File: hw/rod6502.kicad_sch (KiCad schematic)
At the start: 4 parts, among them J1 Conn_01x08_Socket, J2 Conn_01x08_Socket, U1 W65C02SxP

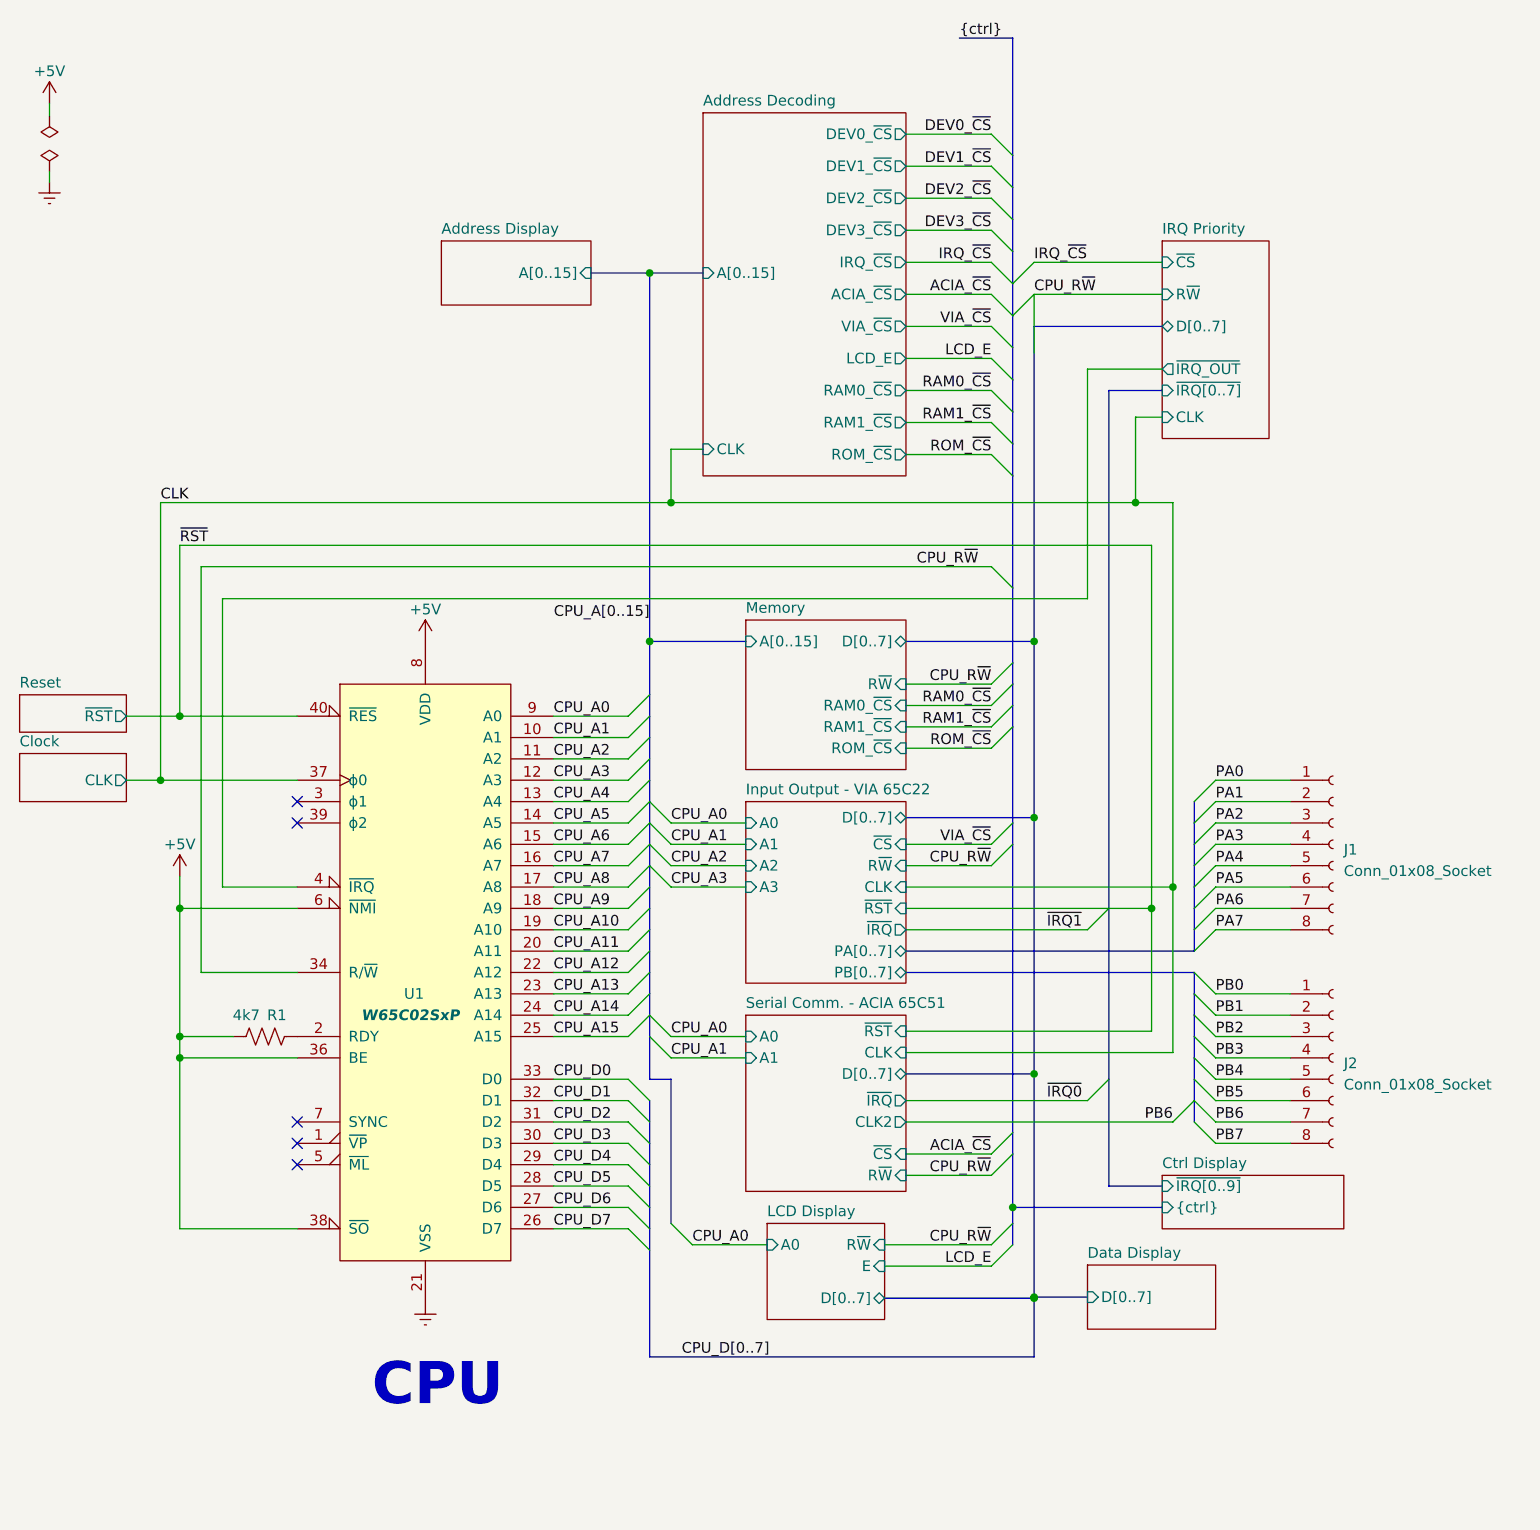
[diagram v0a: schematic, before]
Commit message: add hw design for veraduino
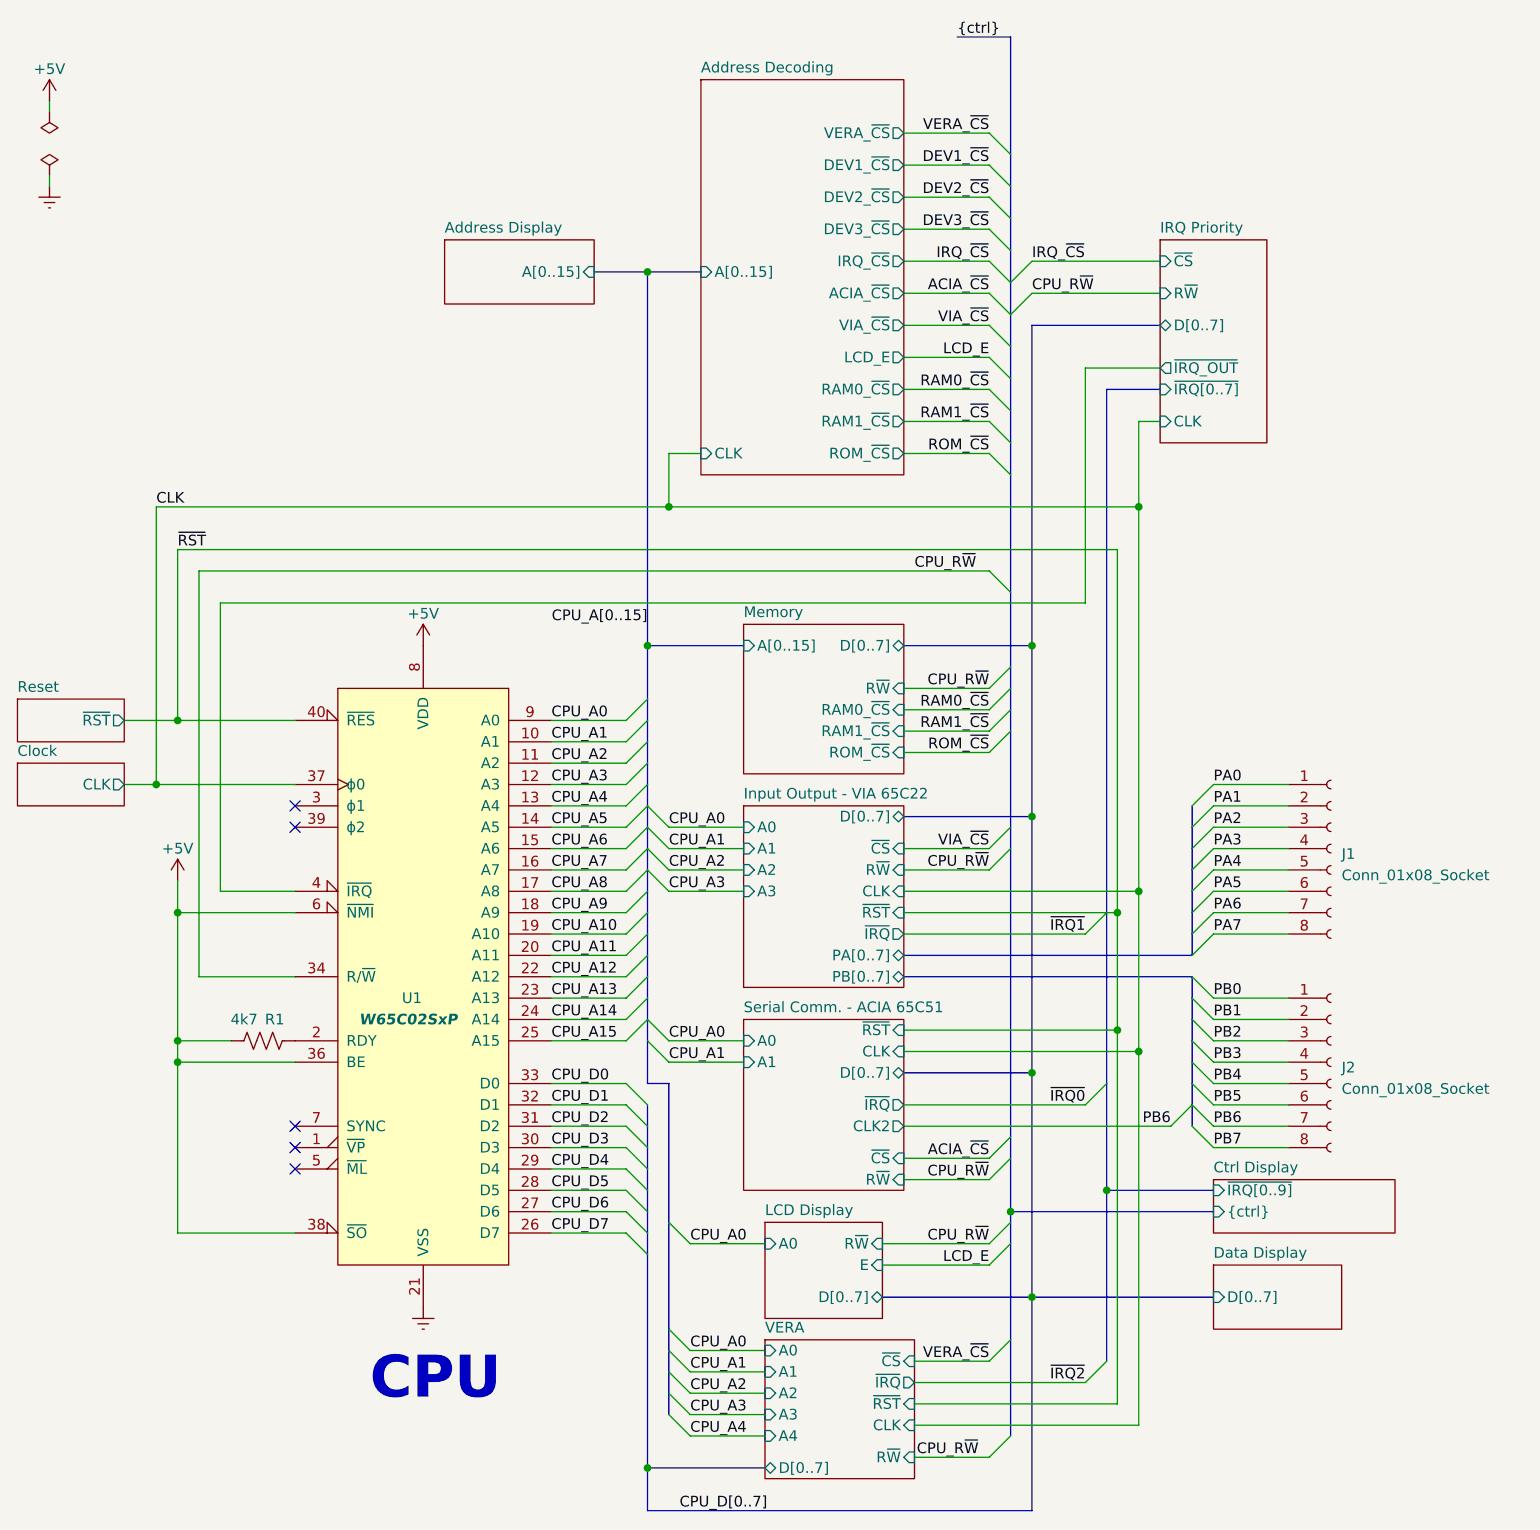
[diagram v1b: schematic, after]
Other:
- added sheet VERA (vera.kicad_sch.kicad_sch)
- sheet Address Decoding ports: added VERA_~{CS}; removed DEV0_~{CS}
- moved on the sheet: J1, J2, R1, U1

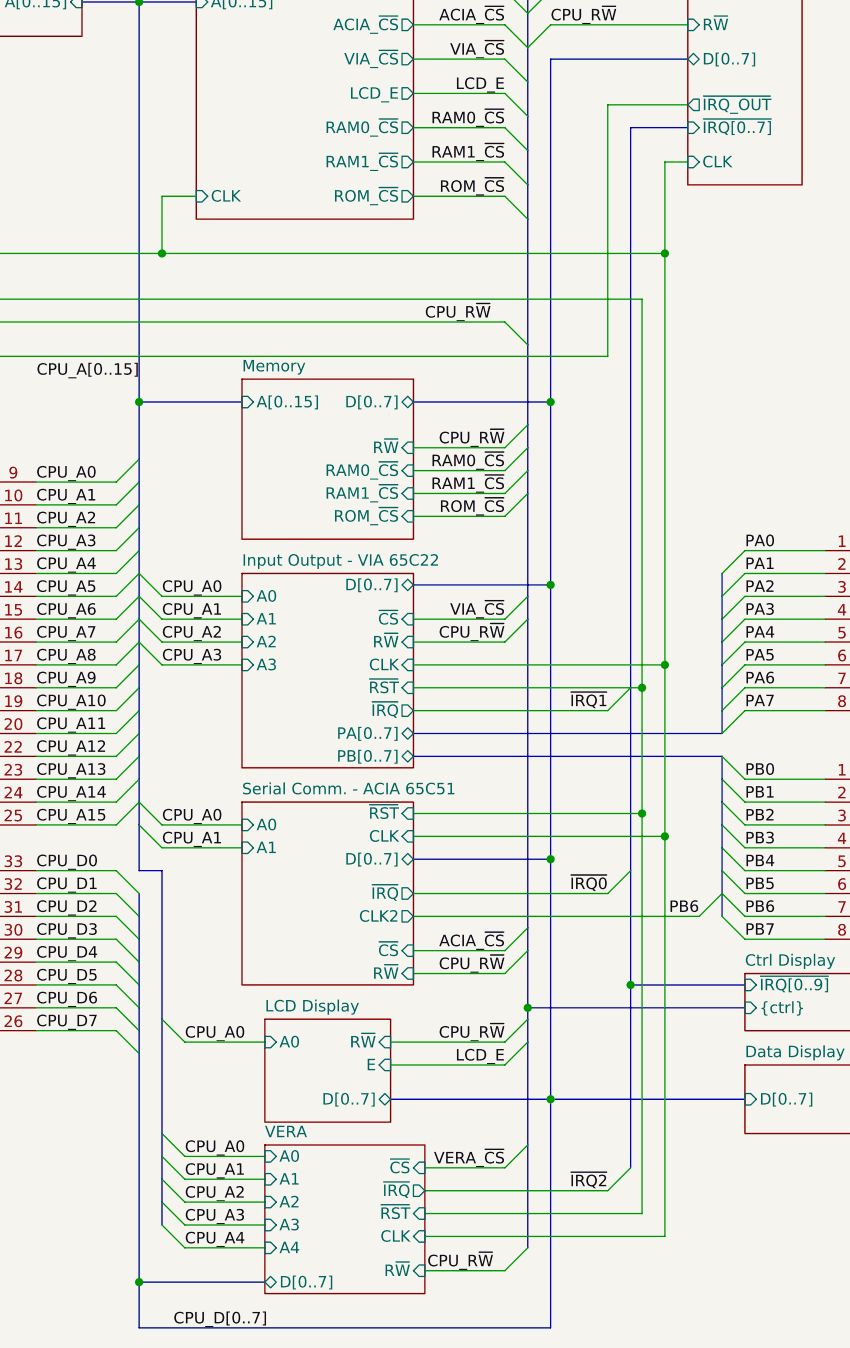
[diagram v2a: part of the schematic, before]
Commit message: clean up hw schematics
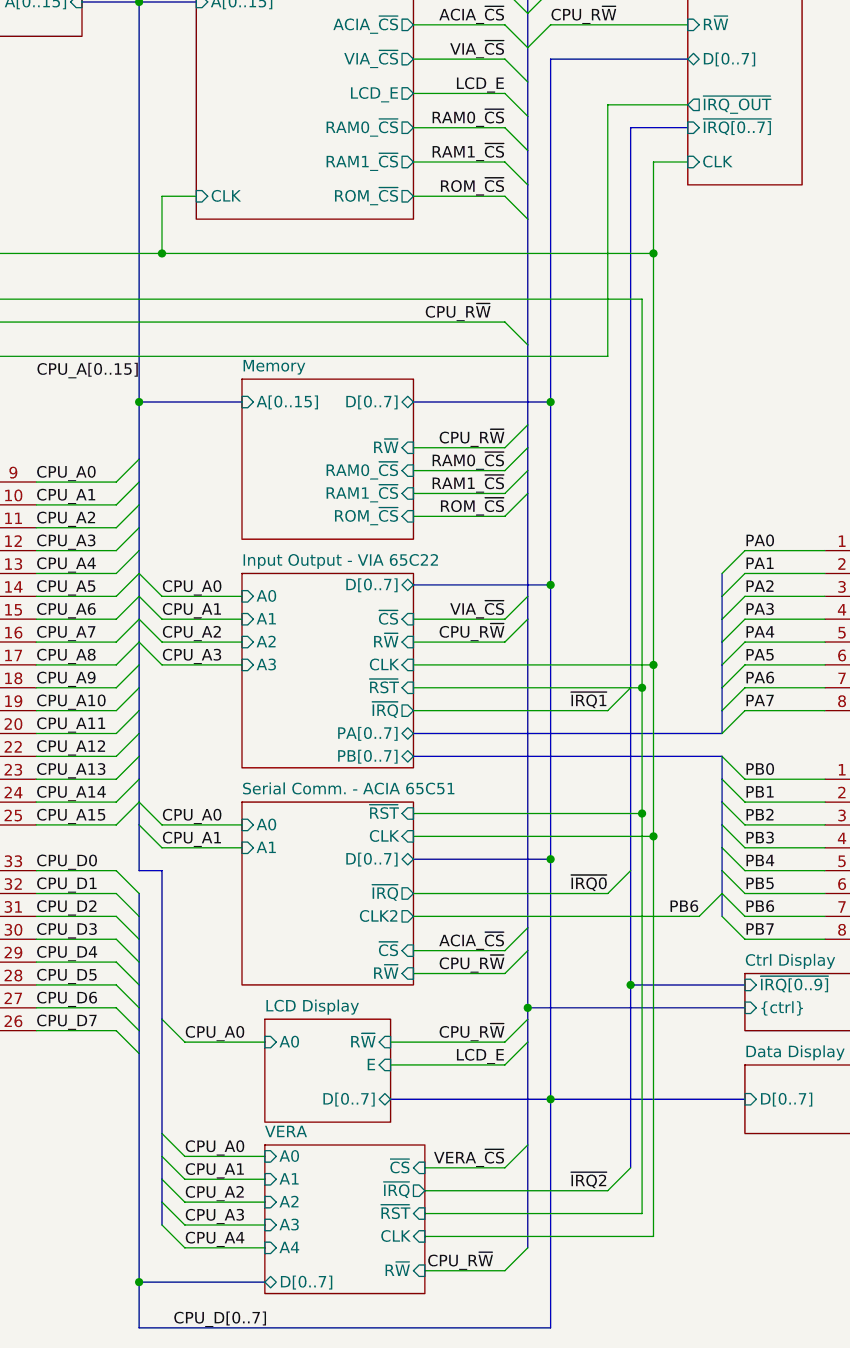
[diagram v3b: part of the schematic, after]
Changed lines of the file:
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@@
   (junction (at 137.16 88.9) (diameter 0) (color 0 0 0 0)
   )
+  (junction (at 148.59 72.39) (diameter 0) (color 0 0 0 0)
+  )
   (junction (at 35.56 120.65) (diameter 0) (color 0 0 0 0)
   )
@@
   (junction (at 91.44 88.9) (diameter 0) (color 0 0 0 0)
   )
+  (junction (at 148.59 118.11) (diameter 0) (color 0 0 0 0)
+  )
   (junction (at 137.16 139.7) (diameter 0) (color 0 0 0 0)
   )
@@
   (junction (at 137.16 166.37) (diameter 0) (color 0 0 0 0)
   )
+  (junction (at 148.59 137.16) (diameter 0) (color 0 0 0 0)
+  )
   (junction (at 147.32 120.65) (diameter 0) (color 0 0 0 0)
-  )
-  (junction (at 149.86 137.16) (diameter 0) (color 0 0 0 0)
-  )
-  (junction (at 149.86 118.11) (diameter 0) (color 0 0 0 0)
-  )
-  (junction (at 149.86 72.39) (diameter 0) (color 0 0 0 0)
   )
   (junction (at 137.16 109.22) (diameter 0) (color 0 0 0 0)
@@
     (stroke (width 0) (type default))
   )
-  (wire (pts (xy 93.98 72.39) (xy 149.86 72.39))
-    (stroke (width 0) (type default))
-  )
-  (wire (pts (xy 149.86 72.39) (xy 149.86 118.11))
+  (wire (pts (xy 93.98 72.39) (xy 148.59 72.39))
+    (stroke (width 0) (type default))
+  )
+  (wire (pts (xy 148.59 72.39) (xy 148.59 118.11))
     (stroke (width 0) (type default))
   )
@@
     (stroke (width 0) (type default))
   )
-  (wire (pts (xy 123.19 181.61) (xy 149.86 181.61))
+  (wire (pts (xy 123.19 181.61) (xy 148.59 181.61))
     (stroke (width 0) (type default))
   )
@@
     (stroke (width 0) (type default))
   )
-  (wire (pts (xy 121.92 118.11) (xy 149.86 118.11))
+  (wire (pts (xy 121.92 118.11) (xy 148.59 118.11))
     (stroke (width 0) (type default))
   )
@@
     (stroke (width 0) (type default))
   )
-  (wire (pts (xy 149.86 62.23) (xy 152.4 62.23))
+  (wire (pts (xy 148.59 62.23) (xy 152.4 62.23))
     (stroke (width 0) (type default))
   )
@@
     (stroke (width 0) (type default))
   )
-  (wire (pts (xy 149.86 137.16) (xy 149.86 181.61))
+  (wire (pts (xy 148.59 137.16) (xy 148.59 181.61))
     (stroke (width 0) (type default))
   )
@@
     (stroke (width 0) (type default))
   )
-  (wire (pts (xy 149.86 62.23) (xy 149.86 72.39))
+  (wire (pts (xy 148.59 62.23) (xy 148.59 72.39))
     (stroke (width 0) (type default))
   )
@@
     (stroke (width 0) (type default))
   )
-  (wire (pts (xy 121.92 137.16) (xy 149.86 137.16))
+  (wire (pts (xy 121.92 137.16) (xy 148.59 137.16))
     (stroke (width 0) (type default))
   )
@@
     (stroke (width 0) (type default))
   )
-  (wire (pts (xy 149.86 118.11) (xy 149.86 137.16))
-    (stroke (width 0) (type default))
-  )
+  (wire (pts (xy 148.59 118.11) (xy 148.59 137.16))
+    (stroke (width 0) (type default))
+  )
